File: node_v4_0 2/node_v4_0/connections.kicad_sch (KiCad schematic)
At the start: 11 parts, among them J4 Conn_02x08_Odd_Even, J5 Conn_02x02_Odd_Even, J6 GNSS_ANT, J7 RF_ANT

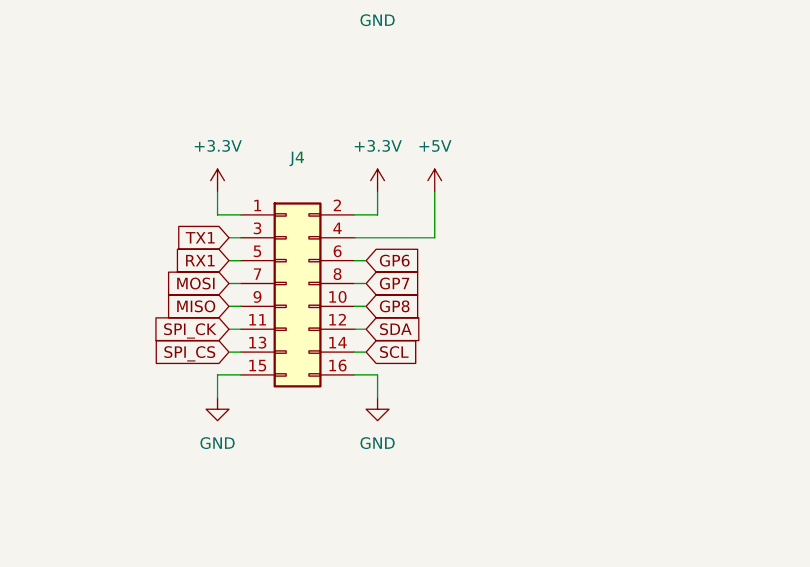
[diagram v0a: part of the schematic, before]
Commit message: most routing done
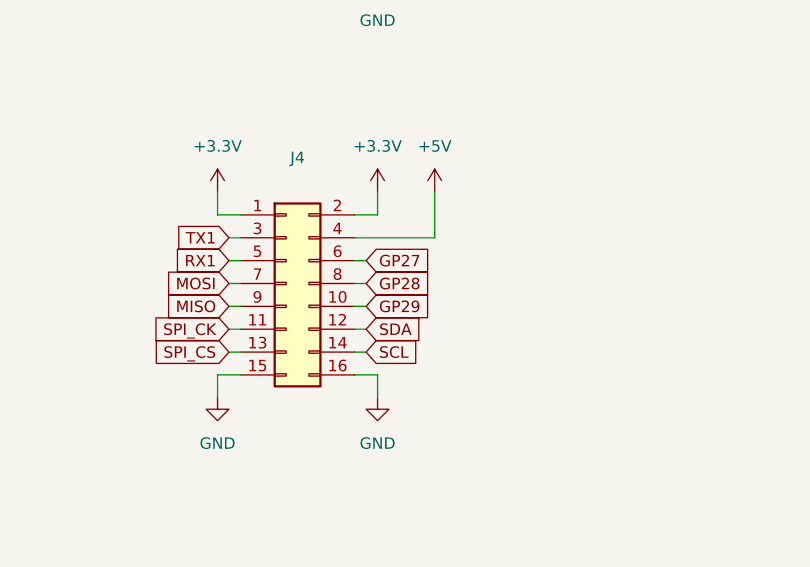
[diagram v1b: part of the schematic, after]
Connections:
- net GP6 renamed GP27
- net GP7 renamed GP28
- net GP8 renamed GP29
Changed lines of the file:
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@@
 		)
 	)
-	(global_label "GP7"
+	(global_label "SCL"
+		(shape input)
+		(at 120.65 107.95 0)
+		(fields_autoplaced yes)
+		(effects
+			(font
+				(size 1.27 1.27)
+			)
+			(justify left)
+		)
+		(property "Intersheetrefs" "${INTERSHEET_REFS}"
+			(at 127.1428 107.95 0)
+			(effects
+				(font
+					(size 1.27 1.27)
+				)
+				(justify left)
+				(hide yes)
+			)
+		)
+	)
+	(global_label "MOSI"
+		(shape input)
+		(at 105.41 100.33 180)
+		(fields_autoplaced yes)
+		(effects
+			(font
+				(size 1.27 1.27)
+			)
+			(justify right)
+		)
+		(property "Intersheetrefs" "${INTERSHEET_REFS}"
+			(at 97.8286 100.33 0)
+			(effects
+				(font
+					(size 1.27 1.27)
+				)
+				(justify right)
+				(hide yes)
+			)
+		)
+	)
+	(global_label "SWD"
+		(shape input)
+		(at 105.41 64.77 180)
+		(fields_autoplaced yes)
+		(effects
+			(font
+				(size 1.27 1.27)
+			)
+			(justify right)
+		)
+		(property "Intersheetrefs" "${INTERSHEET_REFS}"
+			(at 98.4939 64.77 0)
+			(effects
+				(font
+					(size 1.27 1.27)
+				)
+				(justify right)
+				(hide yes)
+			)
+		)
+	)
+	(global_label "MISO"
+		(shape input)
+		(at 105.41 102.87 180)
+		(fields_autoplaced yes)
+		(effects
+			(font
+				(size 1.27 1.27)
+			)
+			(justify right)
+		)
+		(property "Intersheetrefs" "${INTERSHEET_REFS}"
+			(at 97.8286 102.87 0)
+			(effects
+				(font
+					(size 1.27 1.27)
+				)
+				(justify right)
+				(hide yes)
+			)
+		)
+	)
+	(global_label "GNSS_ANT"
+		(shape input)
+		(at 185.42 78.74 180)
+		(fields_autoplaced yes)
+		(effects
+			(font
+				(size 1.27 1.27)
+			)
+			(justify right)
+		)
+		(property "Intersheetrefs" "${INTERSHEET_REFS}"
+			(at 173.061 78.74 0)
+			(effects
+				(font
+					(size 1.27 1.27)
+				)
+				(justify right)
+				(hide yes)
+			)
+		)
+	)
+	(global_label "SPI_CS"
+		(shape input)
+		(at 105.41 107.95 180)
+		(fields_autoplaced yes)
+		(effects
+			(font
+				(size 1.27 1.27)
+			)
+			(justify right)
+		)
+		(property "Intersheetrefs" "${INTERSHEET_REFS}"
+			(at 95.8934 107.95 0)
+			(effects
+				(font
+					(size 1.27 1.27)
+				)
+				(justify right)
+				(hide yes)
+			)
+		)
+	)
+	(global_label "RF_ANT"
+		(shape input)
+		(at 196.85 121.92 180)
+		(fields_autoplaced yes)
+		(effects
+			(font
+				(size 1.27 1.27)
+			)
+			(justify right)
+		)
+		(property "Intersheetrefs" "${INTERSHEET_REFS}"
+			(at 187.1519 121.92 0)
+			(effects
+				(font
+					(size 1.27 1.27)
+				)
+				(justify right)
+				(hide yes)
+			)
+		)
+	)
+	(global_label "TX1"
+		(shape input)
+		(at 105.41 95.25 180)
+		(fields_autoplaced yes)
+		(effects
+			(font
+				(size 1.27 1.27)
+			)
+			(justify right)
+		)
+		(property "Intersheetrefs" "${INTERSHEET_REFS}"
+			(at 99.0382 95.25 0)
+			(effects
+				(font
+					(size 1.27 1.27)
+				)
+				(justify right)
+				(hide yes)
+			)
+		)
+	)
+	(global_label "GP28"
 		(shape input)
 		(at 120.65 100.33 0)
@@
 		)
 		(property "Intersheetrefs" "${INTERSHEET_REFS}"
-			(at 127.3847 100.33 0)
-			(effects
-				(font
-					(size 1.27 1.27)
-				)
-				(justify left)
-				(hide yes)
-			)
-		)
-	)
-	(global_label "GP6"
+			(at 128.5942 100.33 0)
+			(effects
+				(font
+					(size 1.27 1.27)
+				)
+				(justify left)
+				(hide yes)
+			)
+		)
+	)
+	(global_label "GP29"
+		(shape input)
+		(at 120.65 102.87 0)
+		(fields_autoplaced yes)
+		(effects
+			(font
+				(size 1.27 1.27)
+			)
+			(justify left)
+		)
+		(property "Intersheetrefs" "${INTERSHEET_REFS}"
+			(at 128.5942 102.87 0)
+			(effects
+				(font
+					(size 1.27 1.27)
+				)
+				(justify left)
+				(hide yes)
+			)
+		)
+	)
+	(global_label "SDA"
+		(shape input)
+		(at 120.65 105.41 0)
+		(fields_autoplaced yes)
+		(effects
+			(font
+				(size 1.27 1.27)
+			)
+			(justify left)
+		)
+		(property "Intersheetrefs" "${INTERSHEET_REFS}"
+			(at 127.2033 105.41 0)
+			(effects
+				(font
+					(size 1.27 1.27)
+				)
+				(justify left)
+				(hide yes)
+			)
+		)
+	)
+	(global_label "GP27"
 		(shape input)
 		(at 120.65 97.79 0)
@@
 		)
 		(property "Intersheetrefs" "${INTERSHEET_REFS}"
-			(at 127.3847 97.79 0)
-			(effects
-				(font
-					(size 1.27 1.27)
-				)
-				(justify left)
-				(hide yes)
-			)
-		)
-	)
-	(global_label "SCL"
-		(shape input)
-		(at 120.65 107.95 0)
-		(fields_autoplaced yes)
-		(effects
-			(font
-				(size 1.27 1.27)
-			)
-			(justify left)
-		)
-		(property "Intersheetrefs" "${INTERSHEET_REFS}"
-			(at 127.1428 107.95 0)
-			(effects
-				(font
-					(size 1.27 1.27)
-				)
-				(justify left)
-				(hide yes)
-			)
-		)
-	)
-	(global_label "MOSI"
-		(shape input)
-		(at 105.41 100.33 180)
-		(fields_autoplaced yes)
-		(effects
-			(font
-				(size 1.27 1.27)
-			)
-			(justify right)
-		)
-		(property "Intersheetrefs" "${INTERSHEET_REFS}"
-			(at 97.8286 100.33 0)
-			(effects
-				(font
-					(size 1.27 1.27)
-				)
-				(justify right)
-				(hide yes)
-			)
-		)
-	)
-	(global_label "SWD"
-		(shape input)
-		(at 105.41 64.77 180)
-		(fields_autoplaced yes)
-		(effects
-			(font
-				(size 1.27 1.27)
-			)
-			(justify right)
-		)
-		(property "Intersheetrefs" "${INTERSHEET_REFS}"
-			(at 98.4939 64.77 0)
-			(effects
-				(font
-					(size 1.27 1.27)
-				)
-				(justify right)
-				(hide yes)
-			)
-		)
-	)
-	(global_label "MISO"
-		(shape input)
-		(at 105.41 102.87 180)
-		(fields_autoplaced yes)
-		(effects
-			(font
-				(size 1.27 1.27)
-			)
-			(justify right)
-		)
-		(property "Intersheetrefs" "${INTERSHEET_REFS}"
-			(at 97.8286 102.87 0)
-			(effects
-				(font
-					(size 1.27 1.27)
-				)
-				(justify right)
-				(hide yes)
-			)
-		)
-	)
-	(global_label "GNSS_ANT"
-		(shape input)
-		(at 185.42 78.74 180)
-		(fields_autoplaced yes)
-		(effects
-			(font
-				(size 1.27 1.27)
-			)
-			(justify right)
-		)
-		(property "Intersheetrefs" "${INTERSHEET_REFS}"
-			(at 173.061 78.74 0)
-			(effects
-				(font
-					(size 1.27 1.27)
-				)
-				(justify right)
-				(hide yes)
-			)
-		)
-	)
-	(global_label "SPI_CS"
-		(shape input)
-		(at 105.41 107.95 180)
-		(fields_autoplaced yes)
-		(effects
-			(font
-				(size 1.27 1.27)
-			)
-			(justify right)
-		)
-		(property "Intersheetrefs" "${INTERSHEET_REFS}"
-			(at 95.8934 107.95 0)
-			(effects
-				(font
-					(size 1.27 1.27)
-				)
-				(justify right)
-				(hide yes)
-			)
-		)
-	)
-	(global_label "RF_ANT"
-		(shape input)
-		(at 196.85 121.92 180)
-		(fields_autoplaced yes)
-		(effects
-			(font
-				(size 1.27 1.27)
-			)
-			(justify right)
-		)
-		(property "Intersheetrefs" "${INTERSHEET_REFS}"
-			(at 187.1519 121.92 0)
-			(effects
-				(font
-					(size 1.27 1.27)
-				)
-				(justify right)
-				(hide yes)
-			)
-		)
-	)
-	(global_label "TX1"
-		(shape input)
-		(at 105.41 95.25 180)
-		(fields_autoplaced yes)
-		(effects
-			(font
-				(size 1.27 1.27)
-			)
-			(justify right)
-		)
-		(property "Intersheetrefs" "${INTERSHEET_REFS}"
-			(at 99.0382 95.25 0)
-			(effects
-				(font
-					(size 1.27 1.27)
-				)
-				(justify right)
-				(hide yes)
-			)
-		)
-	)
-	(global_label "GP8"
-		(shape input)
-		(at 120.65 102.87 0)
-		(fields_autoplaced yes)
-		(effects
-			(font
-				(size 1.27 1.27)
-			)
-			(justify left)
-		)
-		(property "Intersheetrefs" "${INTERSHEET_REFS}"
-			(at 127.3847 102.87 0)
-			(effects
-				(font
-					(size 1.27 1.27)
-				)
-				(justify left)
-				(hide yes)
-			)
-		)
-	)
-	(global_label "SDA"
-		(shape input)
-		(at 120.65 105.41 0)
-		(fields_autoplaced yes)
-		(effects
-			(font
-				(size 1.27 1.27)
-			)
-			(justify left)
-		)
-		(property "Intersheetrefs" "${INTERSHEET_REFS}"
-			(at 127.2033 105.41 0)
-			(effects
-				(font
+			(at 128.5942 97.79 0)
+			(effects
+				(font
